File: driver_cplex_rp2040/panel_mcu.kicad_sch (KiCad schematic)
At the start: 23 parts, among them SW1 SW_Push, SW2 SW_Push, U2 RP2040, U3 W25Q16JVUXIQ_TR, Y1 12MHz

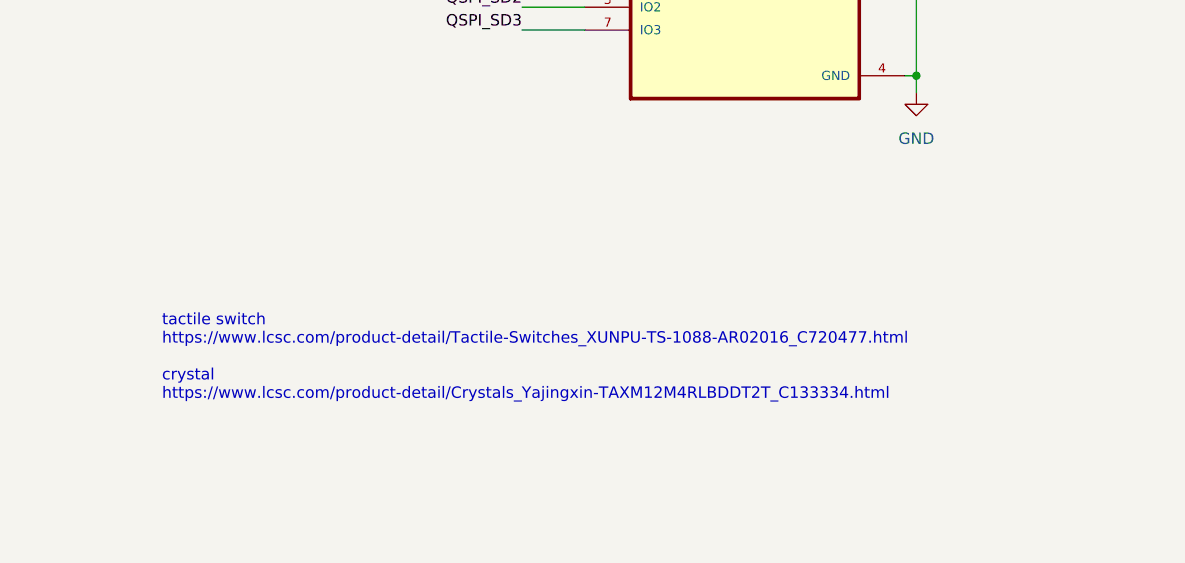
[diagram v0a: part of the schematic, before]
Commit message: Worked on layout.
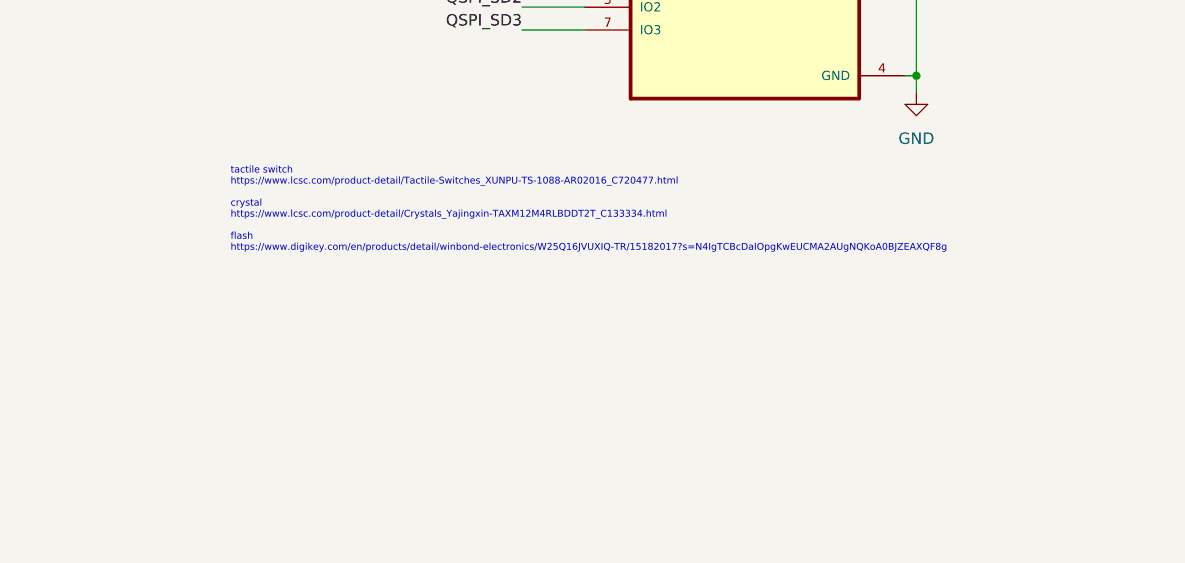
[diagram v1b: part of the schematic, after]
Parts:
- U3: footprint panel_custom:PSON50P300X200X60-9N -> panel_custom:flashmem_PSON50P300X200X60-9N
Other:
- note added: "tactile switch https://www.lcsc.com/product-detail/Tactile-Switches_XUNPU-TS-1088-AR02016_C720477.html crystal https://www.lcsc.com/product-detail/Crystals_Yajingxin-TAXM12M4RLBDDT2T_C133334.html flash https://www.digikey.com/en/products/detail/winbond-electronics/W25Q16JVUXIQ-TR/15182017?s=N4IgTCBcDaIOpgKwEUCMA2AUgNQKoA0BJZEAXQF8g"
- note removed: "tactile switch https://www.lcsc.com/product-detail/Tactile-Switches_XUNPU-TS-1088-AR02016_C720477.html crystal https://www.lcsc.com/product-detail/Crystals_Yajingxin-TAXM12M4RLBDDT2T_C133334.html"
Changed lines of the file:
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@@
     (effects (font (size 2.54 2.54) (thickness 0.508) bold) (justify left bottom))
   )
-  (text "tactile switch\nhttps://www.lcsc.com/product-detail/Tactile-Switches_XUNPU-TS-1088-AR02016_C720477.html\n\ncrystal\nhttps://www.lcsc.com/product-detail/Crystals_Yajingxin-TAXM12M4RLBDDT2T_C133334.html"
-    (at 182.245 151.13 0)
-    (effects (font (size 1.27 1.27)) (justify left bottom))
+  (text "tactile switch\nhttps://www.lcsc.com/product-detail/Tactile-Switches_XUNPU-TS-1088-AR02016_C720477.html\n\ncrystal\nhttps://www.lcsc.com/product-detail/Crystals_Yajingxin-TAXM12M4RLBDDT2T_C133334.html\n\nflash\nhttps://www.digikey.com/en/products/detail/winbond-electronics/W25Q16JVUXIQ-TR/15182017?s=N4IgTCBcDaIOpgKwEUCMA2AUgNQKoA0BJZEAXQF8g"
+    (at 189.865 134.62 0)
+    (effects (font (size 0.762 0.762)) (justify left bottom))
   )
   (label "QSPI_SD2" (at 74.295 103.505 180) (fields_autoplaced)
@@
       (effects (font (size 1.27 1.27)))
     )
-    (property "Footprint" "panel_custom:PSON50P300X200X60-9N" (at 247.015 102.235 0)
+    (property "Footprint" "panel_custom:flashmem_PSON50P300X200X60-9N" (at 247.015 102.235 0)
       (effects (font (size 1.27 1.27)) (justify bottom) hide)
     )

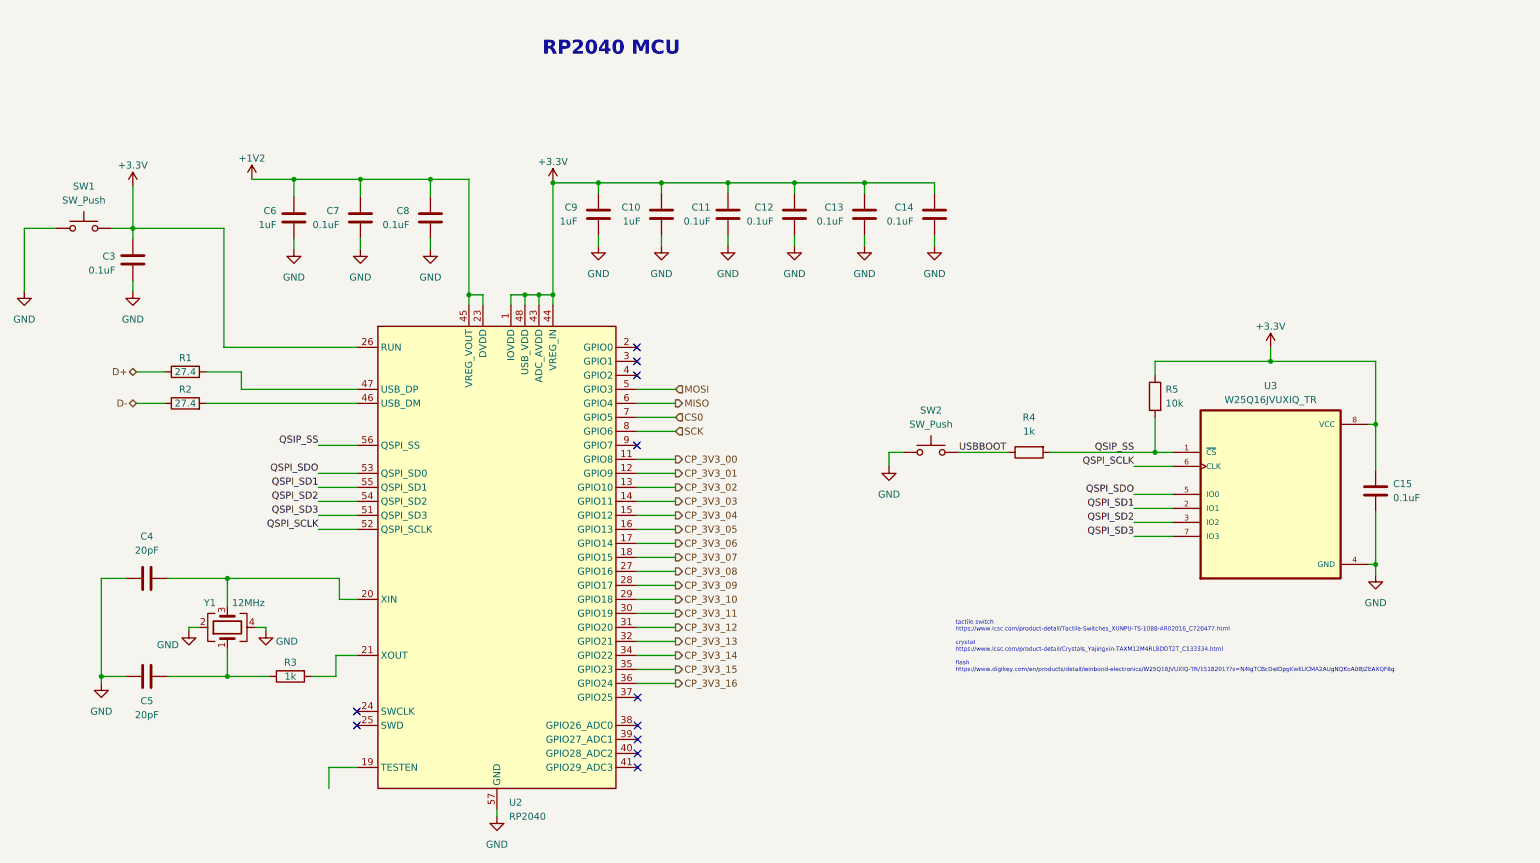
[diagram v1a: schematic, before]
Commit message: Worked on rp2040 cplex layout.
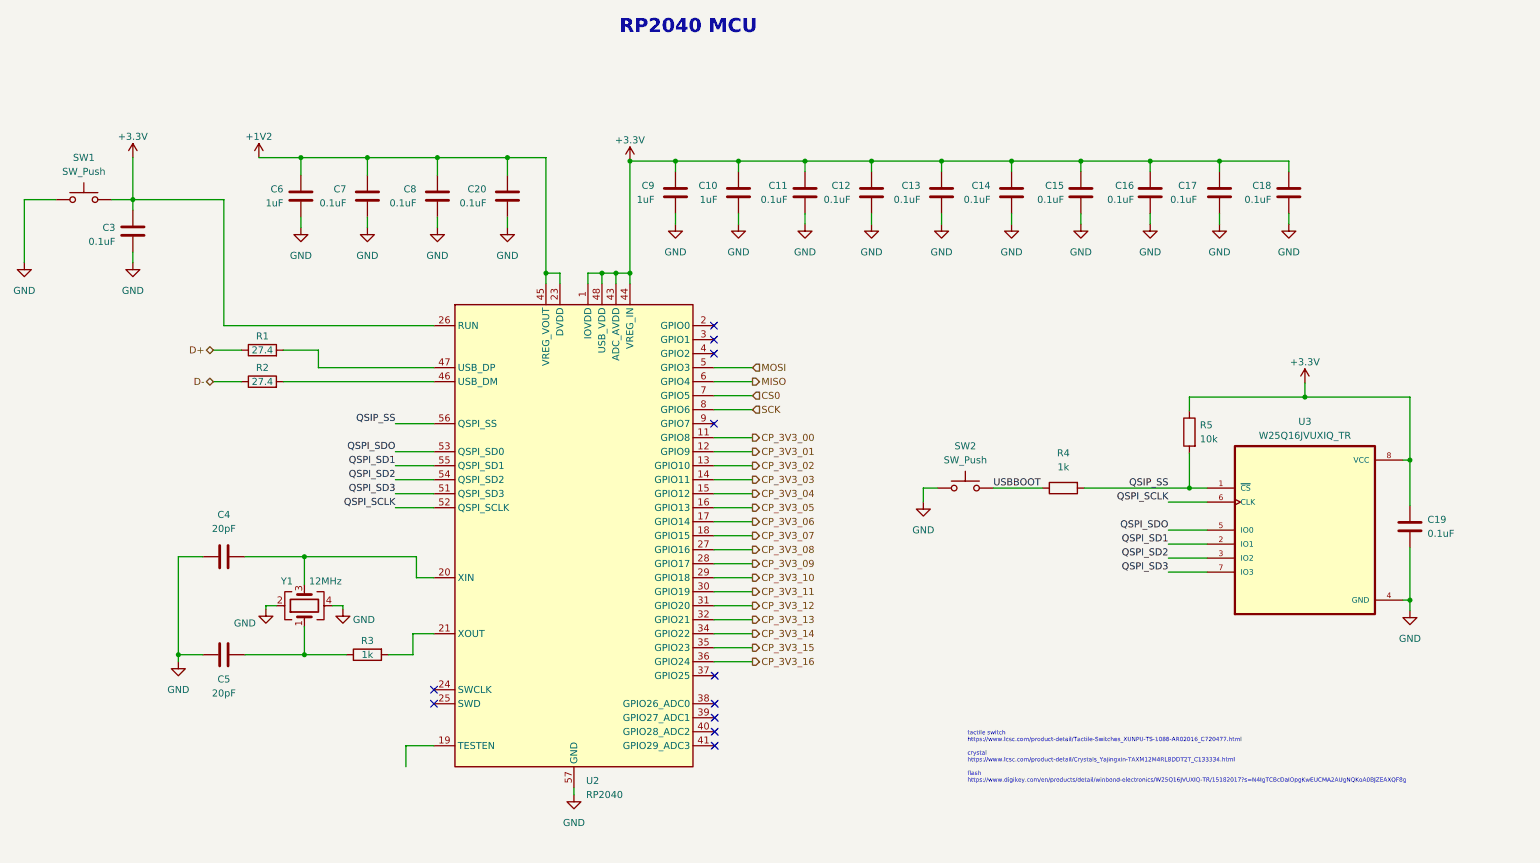
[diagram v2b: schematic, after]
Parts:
- added C15, C16, C17, C18, C20: 0.1uF, panel_custom:C_0201_0603Metric, symbol Device:C
- renumbered C15 to C19
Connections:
- net +1V2: now also C20.2
- net +3.3V: now also C15.2, C16.2, C17.2, C18.2
- net GND: now also C15.1, C16.1, C17.1, C18.1, C20.1
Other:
- moved on the sheet: C10, C11, C12, C13, C14, C19, C3, C4, C5, C6, C7, C8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
